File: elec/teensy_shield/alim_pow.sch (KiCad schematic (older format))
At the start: 0 parts

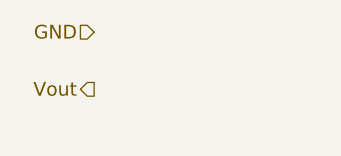
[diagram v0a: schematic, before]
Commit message: Completed new board schematics.
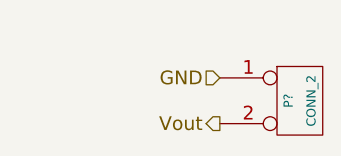
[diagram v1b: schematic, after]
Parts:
- added P?: CONN_2, symbol CONN_2
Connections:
- net GND: now also P?.1 (P1)
- net Vout: now also P?.2 (PM)
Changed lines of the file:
@@
 LIBS:contrib
 LIBS:valves
+LIBS:arduino_shieldsNCL
+LIBS:teensy
+LIBS:pololu
+LIBS:teensy_shield-cache
 EELAYER 24 0
 EELAYER END
 $Descr A4 11693 8268
 encoding utf-8
-Sheet 25 26
+Sheet 25 34
 Title ""
 Date ""
@@
 Comment4 ""
 $EndDescr
-Text HLabel 4600 2700 0    60   Input ~ 0
+Text HLabel 5150 2900 0    60   Input ~ 0
 GND
-Text HLabel 4600 2950 0    60   Output ~ 0
+Text HLabel 5150 3100 0    60   Output ~ 0
 Vout
+$Comp
+L CONN_2 P?
+U 1 1 55E856F0
+P 5500 3000
+F 0 "P?" V 5450 3000 40  0000 C CNN
+F 1 "CONN_2" V 5550 3000 40  0000 C CNN
+F 2 "" H 5500 3000 60  0000 C CNN
+F 3 "" H 5500 3000 60  0000 C CNN
+	1    5500 3000
+	1    0    0    -1
+$EndComp
 $EndSCHEMATC
